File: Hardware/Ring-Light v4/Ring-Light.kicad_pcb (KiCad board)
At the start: 4 copper layers, 124 x 135 mm, 134 parts, among them U1 NCR321PASX, U10 NCR321PASX, U11 NCR321PASX, U12 NCR321PASX, U13 NCR321PASX, U14 NCR321PASX, U15 NCR321PASX, U16 NCR321PASX, U17 NCR321PASX, U18 NCR321PASX, U19 NCR321PASX, U2 NCR321PASX, U20 NCR321PASX, U21 NCR321PASX, U22 NCR321PASX, U23 NCR321PASX, U24 NCR321PASX, U25 NCR321PASX, U26 NCR321PASX, U27 NCR321PASX, U28 NCR321PASX, U29 PCA9685BS,118, U3 NCR321PASX, U30 NCR321PASX, U31 NCR321PASX, U32 NCR321PASX, U33 NCR321PASX, U4 NCR321PASX, U5 NCR321PASX, U6 NCR321PASX, U7 NCR321PASX, U8 NCR321PASX, U9 NCR321PASX

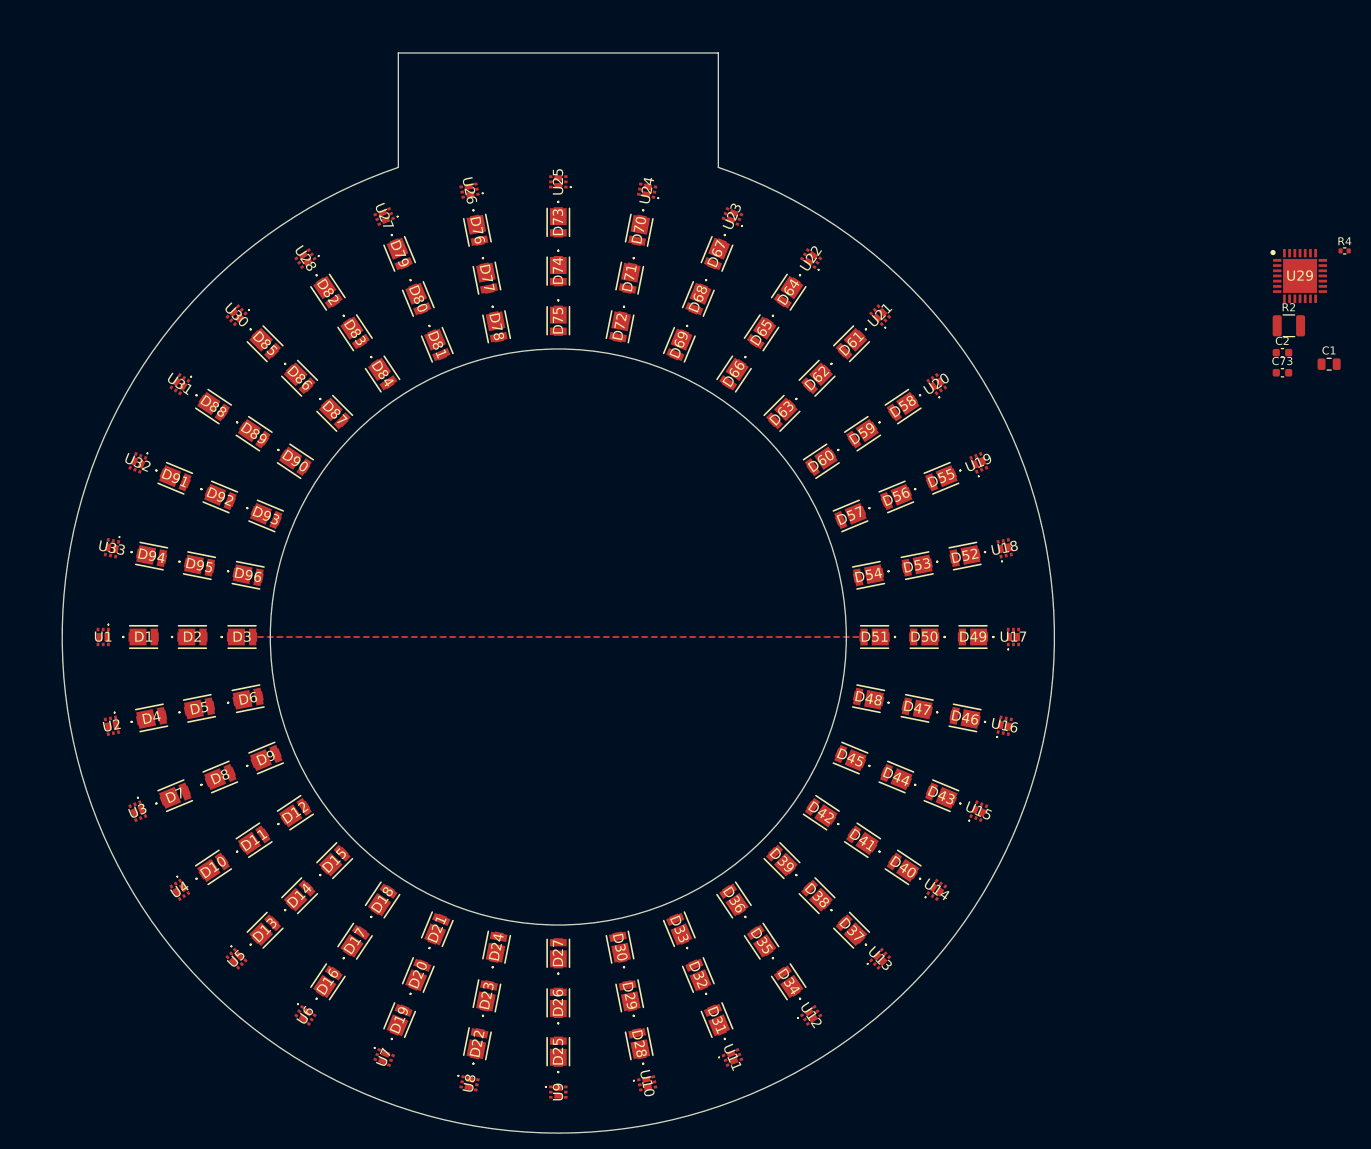
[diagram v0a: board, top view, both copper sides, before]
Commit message: m
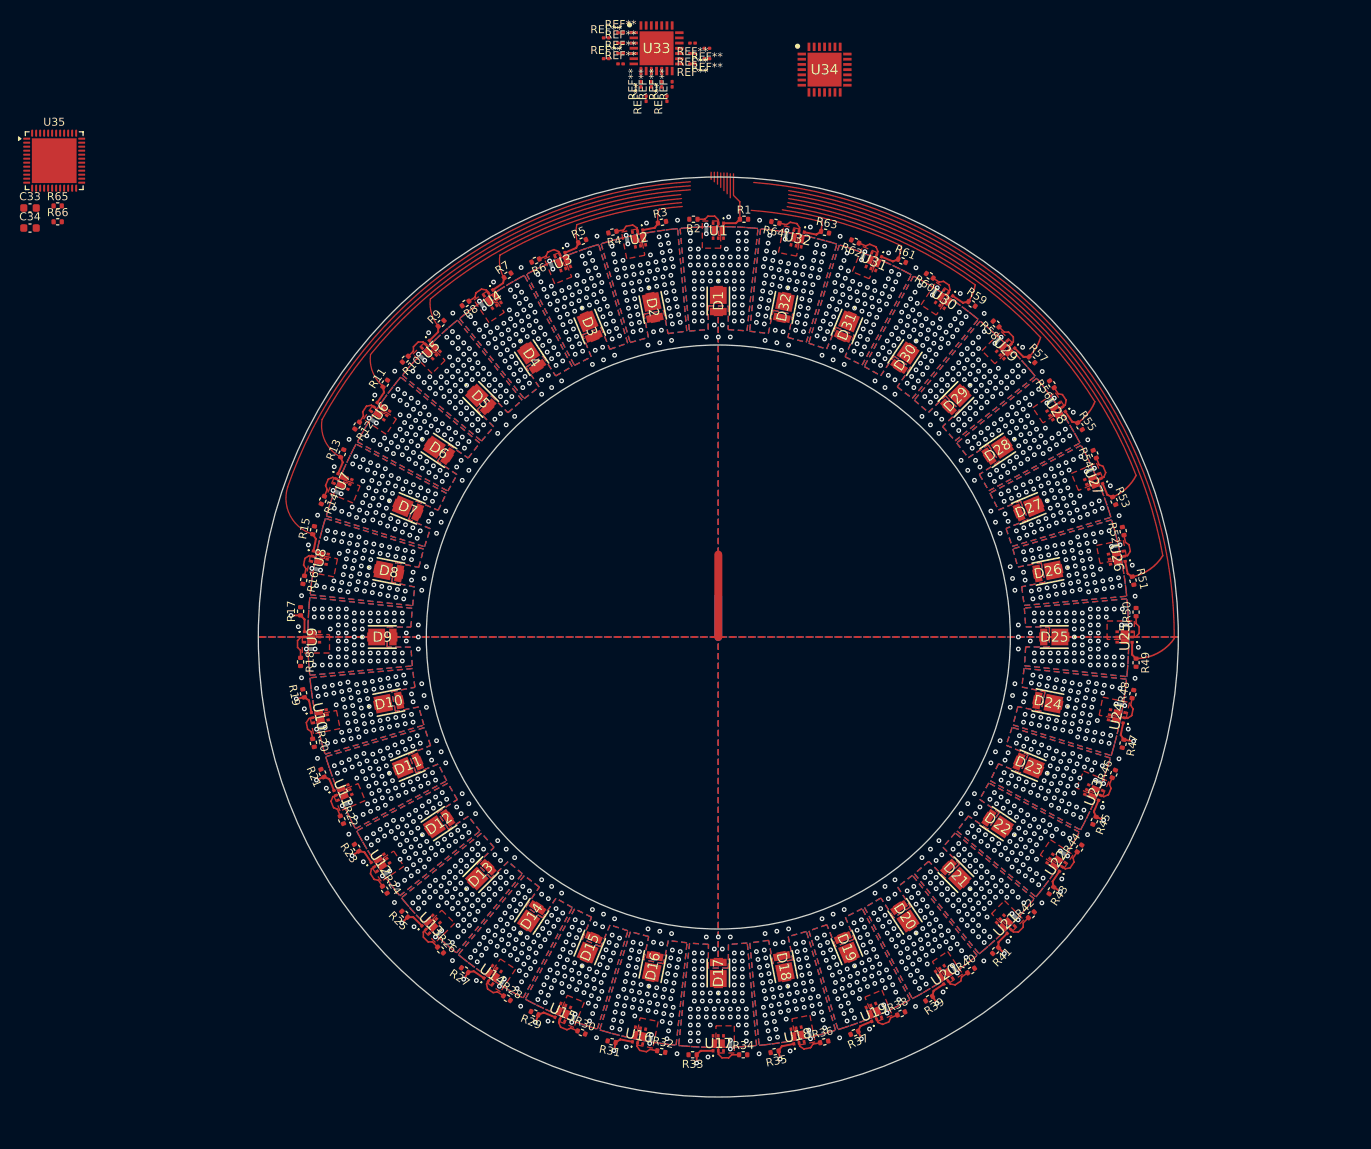
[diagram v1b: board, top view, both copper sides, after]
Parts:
- removed C1: 1uF, Capacitor_SMD:C_0805_2012Metric
- removed C2, C73: 0.1uF, Capacitor_SMD:C_0603_1608Metric
- removed D33, D34, D35, D36, D37, D38, D39, D40, D41, D42, D43, D44, D45, D46, D47, D48, D49, D50, D51, D52, D53, D54, D55, D56, D57, D58, D59, D60, D61, D62, D63, D64, D65, D66, D67, D68, D69, D70, D71, D72, D73, D74, D75, D76, D77, D78, D79, D80, D81, D82, D83, D84, D85, D86, D87, D88, D89, D90, D91, D92, D93, D94, D95, D96: LED, Library:GWJTLRS1EMLVL5XX531
- added C33: 0.1uF, Capacitor_SMD:C_0603_1608Metric, F.Cu at (34.0, 46.4)
- added C34: 0.1uF, Capacitor_SMD:C_0603_1608Metric, F.Cu at (34.0, 48.9)
- added R1: 100k, Resistor_SMD:R_0402_1005Metric, F.Cu at (123.2, 47.8)
- added R10: 9.09, Resistor_SMD:R_0402_1005Metric, F.Cu at (80.9, 65.3)
- added R11: 100k, Resistor_SMD:R_0402_1005Metric, F.Cu at (78.4, 68.3)
- added R12: 9.09, Resistor_SMD:R_0402_1005Metric, F.Cu at (74.9, 73.6)
- added R13: 100k, Resistor_SMD:R_0402_1005Metric, F.Cu at (73.0, 77.1)
- added R14: 9.09, Resistor_SMD:R_0402_1005Metric, F.Cu at (70.6, 82.9)
- added R15: 100k, Resistor_SMD:R_0402_1005Metric, F.Cu at (69.4, 86.7)
- added R16: 9.09, Resistor_SMD:R_0402_1005Metric, F.Cu at (68.2, 92.9)
- added R17: 100k, Resistor_SMD:R_0402_1005Metric, F.Cu at (67.8, 96.8)
- added R18: 9.09, Resistor_SMD:R_0402_1005Metric, F.Cu at (67.8, 103.1)
- added R19: 100k, Resistor_SMD:R_0402_1005Metric, F.Cu at (68.2, 107.0)
- added R20: 9.09, Resistor_SMD:R_0402_1005Metric, F.Cu at (69.4, 113.2)
- added R21: 100k, Resistor_SMD:R_0402_1005Metric, F.Cu at (70.5, 117.0)
- added R22: 9.09, Resistor_SMD:R_0402_1005Metric, F.Cu at (72.9, 122.9)
- added R23: 100k, Resistor_SMD:R_0402_1005Metric, F.Cu at (74.8, 126.3)
- added R24: 9.09, Resistor_SMD:R_0402_1005Metric, F.Cu at (78.3, 131.6)
- added R25: 100k, Resistor_SMD:R_0402_1005Metric, F.Cu at (80.8, 134.7)
- added R26: 9.09, Resistor_SMD:R_0402_1005Metric, F.Cu at (85.3, 139.1)
- added R27: 100k, Resistor_SMD:R_0402_1005Metric, F.Cu at (88.3, 141.6)
- added R28: 9.09, Resistor_SMD:R_0402_1005Metric, F.Cu at (93.6, 145.1)
- added R29: 100k, Resistor_SMD:R_0402_1005Metric, F.Cu at (97.1, 147.0)
- added R3: 100k, Resistor_SMD:R_0402_1005Metric, F.Cu at (113.0, 48.2)
- added R30: 9.09, Resistor_SMD:R_0402_1005Metric, F.Cu at (102.9, 149.4)
- added R31: 100k, Resistor_SMD:R_0402_1005Metric, F.Cu at (106.7, 150.6)
- added R32: 9.09, Resistor_SMD:R_0402_1005Metric, F.Cu at (112.9, 151.8)
- added R33: 100k, Resistor_SMD:R_0402_1005Metric, F.Cu at (116.8, 152.2)
- added R34: 9.09, Resistor_SMD:R_0402_1005Metric, F.Cu at (123.1, 152.2)
- added R35: 100k, Resistor_SMD:R_0402_1005Metric, F.Cu at (127.0, 151.8)
- added R36: 9.09, Resistor_SMD:R_0402_1005Metric, F.Cu at (133.2, 150.6)
- added R37: 100k, Resistor_SMD:R_0402_1005Metric, F.Cu at (137.0, 149.5)
- added R38: 9.09, Resistor_SMD:R_0402_1005Metric, F.Cu at (142.9, 147.1)
- added R39: 100k, Resistor_SMD:R_0402_1005Metric, F.Cu at (146.3, 145.2)
- added R40: 9.09, Resistor_SMD:R_0402_1005Metric, F.Cu at (151.6, 141.7)
- added R41: 100k, Resistor_SMD:R_0402_1005Metric, F.Cu at (154.7, 139.2)
- added R42: 9.09, Resistor_SMD:R_0402_1005Metric, F.Cu at (159.1, 134.7)
- added R43: 100k, Resistor_SMD:R_0402_1005Metric, F.Cu at (161.6, 131.7)
- added R44: 9.09, Resistor_SMD:R_0402_1005Metric, F.Cu at (165.1, 126.4)
- added R45: 100k, Resistor_SMD:R_0402_1005Metric, F.Cu at (167.0, 122.9)
- added R46: 9.09, Resistor_SMD:R_0402_1005Metric, F.Cu at (169.4, 117.1)
- added R47: 100k, Resistor_SMD:R_0402_1005Metric, F.Cu at (170.6, 113.3)
- added R48: 9.09, Resistor_SMD:R_0402_1005Metric, F.Cu at (171.8, 107.1)
- added R49: 100k, Resistor_SMD:R_0402_1005Metric, F.Cu at (172.2, 103.2)
- added R5: 100k, Resistor_SMD:R_0402_1005Metric, F.Cu at (103.0, 50.5)
- added R50: 9.09, Resistor_SMD:R_0402_1005Metric, F.Cu at (172.2, 96.9)
- added R51: 100k, Resistor_SMD:R_0402_1005Metric, F.Cu at (171.8, 93.0)
- added R52: 9.09, Resistor_SMD:R_0402_1005Metric, F.Cu at (170.6, 86.8)
- added R53: 100k, Resistor_SMD:R_0402_1005Metric, F.Cu at (169.5, 83.0)
- added R54: 9.09, Resistor_SMD:R_0402_1005Metric, F.Cu at (167.1, 77.1)
- added R55: 100k, Resistor_SMD:R_0402_1005Metric, F.Cu at (165.2, 73.7)
- added R56: 9.09, Resistor_SMD:R_0402_1005Metric, F.Cu at (161.7, 68.4)
- added R57: 100k, Resistor_SMD:R_0402_1005Metric, F.Cu at (159.2, 65.3)
- added R58: 9.09, Resistor_SMD:R_0402_1005Metric, F.Cu at (154.7, 60.9)
- added R59: 100k, Resistor_SMD:R_0402_1005Metric, F.Cu at (151.7, 58.4)
- added R6: 9.09, Resistor_SMD:R_0402_1005Metric, F.Cu at (97.1, 52.9)
- added R60: 9.09, Resistor_SMD:R_0402_1005Metric, F.Cu at (146.4, 54.9)
- added R61: 100k, Resistor_SMD:R_0402_1005Metric, F.Cu at (142.9, 53.0)
- added R62: 9.09, Resistor_SMD:R_0402_1005Metric, F.Cu at (137.1, 50.6)
- added R63: 100k, Resistor_SMD:R_0402_1005Metric, F.Cu at (133.3, 49.4)
- added R64: 9.09, Resistor_SMD:R_0402_1005Metric, F.Cu at (127.1, 48.2)
- added R65: 10k, Resistor_SMD:R_0402_1005Metric, F.Cu at (37.4, 46.1)
- added R66: 10k, Resistor_SMD:R_0402_1005Metric, F.Cu at (37.4, 48.1)
- added R7: 100k, Resistor_SMD:R_0402_1005Metric, F.Cu at (93.7, 54.8)
- added R8: 9.09, Resistor_SMD:R_0402_1005Metric, F.Cu at (88.4, 58.3)
- added R9: 100k, Resistor_SMD:R_0402_1005Metric, F.Cu at (85.3, 60.8)
- added REF**: R_0201_0603Metric, Resistor_SMD:R_0201_0603Metric, F.Cu at (118.6, 27.7)
- added REF**: R_0201_0603Metric, Resistor_SMD:R_0201_0603Metric, F.Cu at (110.3, 30.9)
- added REF**: R_0201_0603Metric, Resistor_SMD:R_0201_0603Metric, F.Cu at (106.0, 25.1)
- added REF**: R_0201_0603Metric, Resistor_SMD:R_0201_0603Metric, F.Cu at (116.8, 27.1)
- added REF**: R_0201_0603Metric, Resistor_SMD:R_0201_0603Metric, F.Cu at (116.8, 25.8)
- added REF**: R_0201_0603Metric, Resistor_SMD:R_0201_0603Metric, F.Cu at (116.8, 28.4)
- added REF**: R_0201_0603Metric, Resistor_SMD:R_0201_0603Metric, F.Cu at (111.0, 32.7)
- added REF**: R_0201_0603Metric, Resistor_SMD:R_0201_0603Metric, F.Cu at (118.6, 26.4)
- added REF**: R_0201_0603Metric, Resistor_SMD:R_0201_0603Metric, F.Cu at (113.6, 32.7)
- added REF**: R_0201_0603Metric, Resistor_SMD:R_0201_0603Metric, F.Cu at (111.6, 30.9)
- added REF**: R_0201_0603Metric, Resistor_SMD:R_0201_0603Metric, F.Cu at (107.8, 28.4)
- added REF**: R_0201_0603Metric, Resistor_SMD:R_0201_0603Metric, F.Cu at (106.0, 27.7)
- added REF**: R_0201_0603Metric, Resistor_SMD:R_0201_0603Metric, F.Cu at (107.8, 24.5)
- added REF**: R_0201_0603Metric, Resistor_SMD:R_0201_0603Metric, F.Cu at (112.9, 30.9)
- added REF**: R_0201_0603Metric, Resistor_SMD:R_0201_0603Metric, F.Cu at (107.8, 27.1)
- added REF**: R_0201_0603Metric, Resistor_SMD:R_0201_0603Metric, F.Cu at (107.8, 25.8)
- added REF**: R_0201_0603Metric, Resistor_SMD:R_0201_0603Metric, F.Cu at (114.2, 30.9)
- added U34: PCA9685BS,118, Library:QFN65P600X600X100-29N-D, F.Cu at (133.3, 29.1)
- added U35: STM32WB50CGUx, Package_DFN_QFN:QFN-48-1EP_7x7mm_P0.5mm_EP5.6x5.6mm, F.Cu at (37.0, 40.5)
- R2: value 80.6 -> 9.09; footprint Resistor_SMD:R_1210_3225Metric -> Resistor_SMD:R_0402_1005Metric
- R4: value 10k -> 9.09
- U29: value PCA9685BS,118 -> NCR321PASX; footprint Library:QFN65P600X600X100-29N-D -> Library:NCR321PASX
- U33: value NCR321PASX -> PCA9685BS,118; footprint Library:NCR321PASX -> Library:QFN65P600X600X100-29N-D
- moved U28 95.8 mm to (162.2, 71.8)
- moved U27 94.7 mm to (166.9, 80.6)
- moved U26 93.0 mm to (169.8, 90.1)
- moved U33 92.4 mm to (112.3, 26.4), turned to 0 degrees
- moved U1 92.2 mm to (120.0, 49.2)
- moved R4 91.6 mm to (106.8, 49.4), turned to -168.75 degrees
- moved U25 90.8 mm to (170.8, 100.0)
- moved U2 89.7 mm to (110.1, 50.2)
- moved U30 88.5 mm to (148.2, 57.8), turned to 146.25 degrees
- moved D31 88.2 mm to (136.1, 61.2), turned to -112.5 degrees
- moved U24 88.1 mm to (169.8, 109.9)
- moved U31 88.1 mm to (139.4, 53.1), turned to 157.5 degrees
- moved U32 87.1 mm to (129.9, 50.2), turned to 168.75 degrees
- moved U3 86.8 mm to (100.6, 53.1)
- moved D28 86.7 mm to (154.9, 76.7), turned to -146.25 degrees
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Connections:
- D1 pad 1: Net-(D1-K-Pad1) -> /OUT1
- D1 pad 2: Net-(D1-K-Pad1) -> /OUT1
- D1 pad 3: Net-(D1-A-Pad3) -> +12V
- D1 pad 4: Net-(D1-A-Pad3) -> +12V
- D10 pad 1: Net-(D1-K-Pad1) -> /OUT10
- D10 pad 2: Net-(D1-K-Pad1) -> /OUT10
- D10 pad 3: Net-(D1-A-Pad3) -> +12V
- D10 pad 4: Net-(D1-A-Pad3) -> +12V
- D11 pad 1: Net-(D1-A-Pad3) -> /OUT11
- D11 pad 2: Net-(D1-A-Pad3) -> /OUT11
- D11 pad 3: Net-(D2-A-Pad3) -> +12V
- D11 pad 4: Net-(D2-A-Pad3) -> +12V
- D12 pad 1: Net-(D2-A-Pad3) -> /OUT12
- D12 pad 2: Net-(D2-A-Pad3) -> /OUT12
- D13 pad 1: Net-(D1-K-Pad1) -> /OUT13
- D13 pad 2: Net-(D1-K-Pad1) -> /OUT13
- D13 pad 3: Net-(D1-A-Pad3) -> +12V
- D13 pad 4: Net-(D1-A-Pad3) -> +12V
- D14 pad 1: Net-(D1-A-Pad3) -> /OUT14
- D14 pad 2: Net-(D1-A-Pad3) -> /OUT14
- D14 pad 3: Net-(D2-A-Pad3) -> +12V
- D14 pad 4: Net-(D2-A-Pad3) -> +12V
- D15 pad 1: Net-(D2-A-Pad3) -> /OUT15
- D15 pad 2: Net-(D2-A-Pad3) -> /OUT15
- D16 pad 1: Net-(D1-K-Pad1) -> /OUT16
- D16 pad 2: Net-(D1-K-Pad1) -> /OUT16
- D16 pad 3: Net-(D1-A-Pad3) -> +12V
- D16 pad 4: Net-(D1-A-Pad3) -> +12V
- D17 pad 1: Net-(D1-A-Pad3) -> /OUT17
- D17 pad 2: Net-(D1-A-Pad3) -> /OUT17
- D17 pad 3: Net-(D2-A-Pad3) -> +12V
- D17 pad 4: Net-(D2-A-Pad3) -> +12V
- D18 pad 1: Net-(D2-A-Pad3) -> /OUT18
- D18 pad 2: Net-(D2-A-Pad3) -> /OUT18
- D19 pad 1: Net-(D1-K-Pad1) -> /OUT19
- D19 pad 2: Net-(D1-K-Pad1) -> /OUT19
- D19 pad 3: Net-(D1-A-Pad3) -> +12V
- D19 pad 4: Net-(D1-A-Pad3) -> +12V
- D2 pad 1: Net-(D1-A-Pad3) -> /OUT2
- D2 pad 2: Net-(D1-A-Pad3) -> /OUT2
- D2 pad 3: Net-(D2-A-Pad3) -> +12V
- D2 pad 4: Net-(D2-A-Pad3) -> +12V
- D20 pad 1: Net-(D1-A-Pad3) -> /OUT20
- D20 pad 2: Net-(D1-A-Pad3) -> /OUT20
- D20 pad 3: Net-(D2-A-Pad3) -> +12V
- D20 pad 4: Net-(D2-A-Pad3) -> +12V
- D21 pad 1: Net-(D2-A-Pad3) -> /OUT21
- D21 pad 2: Net-(D2-A-Pad3) -> /OUT21
- D22 pad 1: Net-(D1-K-Pad1) -> /OUT22
- D22 pad 2: Net-(D1-K-Pad1) -> /OUT22
- D22 pad 3: Net-(D1-A-Pad3) -> +12V
- D22 pad 4: Net-(D1-A-Pad3) -> +12V
- D23 pad 1: Net-(D1-A-Pad3) -> /OUT23
- D23 pad 2: Net-(D1-A-Pad3) -> /OUT23
- D23 pad 3: Net-(D2-A-Pad3) -> +12V
- D23 pad 4: Net-(D2-A-Pad3) -> +12V
- D24 pad 1: Net-(D2-A-Pad3) -> /OUT24
- D24 pad 2: Net-(D2-A-Pad3) -> /OUT24
- D25 pad 1: Net-(D1-K-Pad1) -> /OUT25
- D25 pad 2: Net-(D1-K-Pad1) -> /OUT25
- D25 pad 3: Net-(D1-A-Pad3) -> +12V
- D25 pad 4: Net-(D1-A-Pad3) -> +12V
- D26 pad 1: Net-(D1-A-Pad3) -> /OUT26
- D26 pad 2: Net-(D1-A-Pad3) -> /OUT26
- D26 pad 3: Net-(D2-A-Pad3) -> +12V
- D26 pad 4: Net-(D2-A-Pad3) -> +12V
- D27 pad 1: Net-(D2-A-Pad3) -> /OUT27
- D27 pad 2: Net-(D2-A-Pad3) -> /OUT27
- D28 pad 1: Net-(D1-K-Pad1) -> /OUT28
- D28 pad 2: Net-(D1-K-Pad1) -> /OUT28
- D28 pad 3: Net-(D1-A-Pad3) -> +12V
- D28 pad 4: Net-(D1-A-Pad3) -> +12V
- D29 pad 1: Net-(D1-A-Pad3) -> /OUT29
- D29 pad 2: Net-(D1-A-Pad3) -> /OUT29
- D29 pad 3: Net-(D2-A-Pad3) -> +12V
- D29 pad 4: Net-(D2-A-Pad3) -> +12V
- D3 pad 1: Net-(D2-A-Pad3) -> /OUT3
- D3 pad 2: Net-(D2-A-Pad3) -> /OUT3
- D30 pad 1: Net-(D2-A-Pad3) -> /OUT30
- D30 pad 2: Net-(D2-A-Pad3) -> /OUT30
- D31 pad 1: Net-(D1-K-Pad1) -> /OUT31
- D31 pad 2: Net-(D1-K-Pad1) -> /OUT31
- D31 pad 3: Net-(D1-A-Pad3) -> +12V
- D31 pad 4: Net-(D1-A-Pad3) -> +12V
- D32 pad 1: Net-(D1-A-Pad3) -> /OUT32
- D32 pad 2: Net-(D1-A-Pad3) -> /OUT32
- D32 pad 3: Net-(D2-A-Pad3) -> +12V
- D32 pad 4: Net-(D2-A-Pad3) -> +12V
- D4 pad 1: Net-(D1-K-Pad1) -> /OUT4
- D4 pad 2: Net-(D1-K-Pad1) -> /OUT4
- D4 pad 3: Net-(D1-A-Pad3) -> +12V
- D4 pad 4: Net-(D1-A-Pad3) -> +12V
- D5 pad 1: Net-(D1-A-Pad3) -> /OUT5
- D5 pad 2: Net-(D1-A-Pad3) -> /OUT5
- D5 pad 3: Net-(D2-A-Pad3) -> +12V
- D5 pad 4: Net-(D2-A-Pad3) -> +12V
- D6 pad 1: Net-(D2-A-Pad3) -> /OUT6
- D6 pad 2: Net-(D2-A-Pad3) -> /OUT6
- D7 pad 1: Net-(D1-K-Pad1) -> /OUT7
- D7 pad 2: Net-(D1-K-Pad1) -> /OUT7
- D7 pad 3: Net-(D1-A-Pad3) -> +12V
- D7 pad 4: Net-(D1-A-Pad3) -> +12V
- D8 pad 1: Net-(D1-A-Pad3) -> /OUT8
- D8 pad 2: Net-(D1-A-Pad3) -> /OUT8
- D8 pad 3: Net-(D2-A-Pad3) -> +12V
- D8 pad 4: Net-(D2-A-Pad3) -> +12V
- D9 pad 1: Net-(D2-A-Pad3) -> /OUT9
- D9 pad 2: Net-(D2-A-Pad3) -> /OUT9
- R2 pad 1: Net-(U1-REXT) -> /REXT1
- R4 pad 1: SDA -> /REXT2
- R4 pad 2: +3.3V -> GND
- U1 pad 1: +12V -> PWM1
- U1 pad 2: Net-(U1-REXT) -> /REXT1
- U1 pad 6: Net-(D1-K-Pad1) -> /OUT1
- U1 pad 7: Net-(D1-K-Pad1) -> /OUT1
- U10 pad 1: +12V -> PWM10
- U10 pad 2: Net-(U1-REXT) -> /REXT10
- U10 pad 3: unconnected-(U1-N/C_1-Pad3) -> unconnected-(U10-N/C_1-Pad3)
- U10 pad 4: unconnected-(U1-N/C_2-Pad4) -> unconnected-(U10-N/C_2-Pad4)
- U10 pad 6: Net-(D1-K-Pad1) -> /OUT10
- U10 pad 7: Net-(D1-K-Pad1) -> /OUT10
- U10 pad 8: unconnected-(U1-N/C_3-Pad8) -> unconnected-(U10-N/C_3-Pad8)
- U11 pad 1: +12V -> PWM11
- U11 pad 2: Net-(U1-REXT) -> /REXT11
- U11 pad 3: unconnected-(U1-N/C_1-Pad3) -> unconnected-(U11-N/C_1-Pad3)
- U11 pad 4: unconnected-(U1-N/C_2-Pad4) -> unconnected-(U11-N/C_2-Pad4)
- U11 pad 6: Net-(D1-K-Pad1) -> /OUT11
- U11 pad 7: Net-(D1-K-Pad1) -> /OUT11
- U11 pad 8: unconnected-(U1-N/C_3-Pad8) -> unconnected-(U11-N/C_3-Pad8)
- U12 pad 1: +12V -> PWM12
- U12 pad 2: Net-(U1-REXT) -> /REXT12
- U12 pad 3: unconnected-(U1-N/C_1-Pad3) -> unconnected-(U12-N/C_1-Pad3)
- U12 pad 4: unconnected-(U1-N/C_2-Pad4) -> unconnected-(U12-N/C_2-Pad4)
- U12 pad 6: Net-(D1-K-Pad1) -> /OUT12
- U12 pad 7: Net-(D1-K-Pad1) -> /OUT12
- U12 pad 8: unconnected-(U1-N/C_3-Pad8) -> unconnected-(U12-N/C_3-Pad8)
- U13 pad 1: +12V -> PWM13
- U13 pad 2: Net-(U1-REXT) -> /REXT13
- U13 pad 3: unconnected-(U1-N/C_1-Pad3) -> unconnected-(U13-N/C_1-Pad3)
- U13 pad 4: unconnected-(U1-N/C_2-Pad4) -> unconnected-(U13-N/C_2-Pad4)
- U13 pad 6: Net-(D1-K-Pad1) -> /OUT13
- U13 pad 7: Net-(D1-K-Pad1) -> /OUT13
- U13 pad 8: unconnected-(U1-N/C_3-Pad8) -> unconnected-(U13-N/C_3-Pad8)
- U14 pad 1: +12V -> PWM14
- U14 pad 2: Net-(U1-REXT) -> /REXT14
- U14 pad 3: unconnected-(U1-N/C_1-Pad3) -> unconnected-(U14-N/C_1-Pad3)
- U14 pad 4: unconnected-(U1-N/C_2-Pad4) -> unconnected-(U14-N/C_2-Pad4)
- U14 pad 6: Net-(D1-K-Pad1) -> /OUT14
- U14 pad 7: Net-(D1-K-Pad1) -> /OUT14
- U14 pad 8: unconnected-(U1-N/C_3-Pad8) -> unconnected-(U14-N/C_3-Pad8)
- U15 pad 1: +12V -> PWM15
- U15 pad 2: Net-(U1-REXT) -> /REXT15
- U15 pad 3: unconnected-(U1-N/C_1-Pad3) -> unconnected-(U15-N/C_1-Pad3)
- U15 pad 4: unconnected-(U1-N/C_2-Pad4) -> unconnected-(U15-N/C_2-Pad4)
- U15 pad 6: Net-(D1-K-Pad1) -> /OUT15
- U15 pad 7: Net-(D1-K-Pad1) -> /OUT15
- U15 pad 8: unconnected-(U1-N/C_3-Pad8) -> unconnected-(U15-N/C_3-Pad8)
- U16 pad 1: +12V -> PWM16
- U16 pad 2: Net-(U1-REXT) -> /REXT16
- U16 pad 3: unconnected-(U1-N/C_1-Pad3) -> unconnected-(U16-N/C_1-Pad3)
- U16 pad 4: unconnected-(U1-N/C_2-Pad4) -> unconnected-(U16-N/C_2-Pad4)
- U16 pad 6: Net-(D1-K-Pad1) -> /OUT16
- U16 pad 7: Net-(D1-K-Pad1) -> /OUT16
- U16 pad 8: unconnected-(U1-N/C_3-Pad8) -> unconnected-(U16-N/C_3-Pad8)
- U17 pad 1: +12V -> PWM17
- U17 pad 2: Net-(U1-REXT) -> /REXT17
- U17 pad 3: unconnected-(U1-N/C_1-Pad3) -> unconnected-(U17-N/C_1-Pad3)
- U17 pad 4: unconnected-(U1-N/C_2-Pad4) -> unconnected-(U17-N/C_2-Pad4)
- U17 pad 6: Net-(D1-K-Pad1) -> /OUT17
- U17 pad 7: Net-(D1-K-Pad1) -> /OUT17
- U17 pad 8: unconnected-(U1-N/C_3-Pad8) -> unconnected-(U17-N/C_3-Pad8)
- U18 pad 1: +12V -> PWM18
- U18 pad 2: Net-(U1-REXT) -> /REXT18
- U18 pad 3: unconnected-(U1-N/C_1-Pad3) -> unconnected-(U18-N/C_1-Pad3)
- U18 pad 4: unconnected-(U1-N/C_2-Pad4) -> unconnected-(U18-N/C_2-Pad4)
- U18 pad 6: Net-(D1-K-Pad1) -> /OUT18
- U18 pad 7: Net-(D1-K-Pad1) -> /OUT18
- U18 pad 8: unconnected-(U1-N/C_3-Pad8) -> unconnected-(U18-N/C_3-Pad8)
- U19 pad 1: +12V -> PWM19
- U19 pad 2: Net-(U1-REXT) -> /REXT19
- U19 pad 3: unconnected-(U1-N/C_1-Pad3) -> unconnected-(U19-N/C_1-Pad3)
- U19 pad 4: unconnected-(U1-N/C_2-Pad4) -> unconnected-(U19-N/C_2-Pad4)
- U19 pad 6: Net-(D1-K-Pad1) -> /OUT19
- U19 pad 7: Net-(D1-K-Pad1) -> /OUT19
- U19 pad 8: unconnected-(U1-N/C_3-Pad8) -> unconnected-(U19-N/C_3-Pad8)
- U2 pad 1: +12V -> PWM2
- U2 pad 2: Net-(U1-REXT) -> /REXT2
- U2 pad 3: unconnected-(U1-N/C_1-Pad3) -> unconnected-(U2-N/C_1-Pad3)
- U2 pad 4: unconnected-(U1-N/C_2-Pad4) -> unconnected-(U2-N/C_2-Pad4)
- U2 pad 6: Net-(D1-K-Pad1) -> /OUT2
- U2 pad 7: Net-(D1-K-Pad1) -> /OUT2
- U2 pad 8: unconnected-(U1-N/C_3-Pad8) -> unconnected-(U2-N/C_3-Pad8)
- U20 pad 1: +12V -> PWM20
- U20 pad 2: Net-(U1-REXT) -> /REXT20
- U20 pad 3: unconnected-(U1-N/C_1-Pad3) -> unconnected-(U20-N/C_1-Pad3)
- U20 pad 4: unconnected-(U1-N/C_2-Pad4) -> unconnected-(U20-N/C_2-Pad4)
- U20 pad 6: Net-(D1-K-Pad1) -> /OUT20
- U20 pad 7: Net-(D1-K-Pad1) -> /OUT20
- U20 pad 8: unconnected-(U1-N/C_3-Pad8) -> unconnected-(U20-N/C_3-Pad8)
- U21 pad 1: +12V -> PWM21
- U21 pad 2: Net-(U1-REXT) -> /REXT21
- U21 pad 3: unconnected-(U1-N/C_1-Pad3) -> unconnected-(U21-N/C_1-Pad3)
- U21 pad 4: unconnected-(U1-N/C_2-Pad4) -> unconnected-(U21-N/C_2-Pad4)
- U21 pad 6: Net-(D1-K-Pad1) -> /OUT21
- U21 pad 7: Net-(D1-K-Pad1) -> /OUT21
- U21 pad 8: unconnected-(U1-N/C_3-Pad8) -> unconnected-(U21-N/C_3-Pad8)
- U22 pad 1: +12V -> PWM22
- U22 pad 2: Net-(U1-REXT) -> /REXT22
- U22 pad 3: unconnected-(U1-N/C_1-Pad3) -> unconnected-(U22-N/C_1-Pad3)
- U22 pad 4: unconnected-(U1-N/C_2-Pad4) -> unconnected-(U22-N/C_2-Pad4)
- U22 pad 6: Net-(D1-K-Pad1) -> /OUT22
- U22 pad 7: Net-(D1-K-Pad1) -> /OUT22
- U22 pad 8: unconnected-(U1-N/C_3-Pad8) -> unconnected-(U22-N/C_3-Pad8)
- U23 pad 1: +12V -> PWM23
- U23 pad 2: Net-(U1-REXT) -> /REXT23
- U23 pad 3: unconnected-(U1-N/C_1-Pad3) -> unconnected-(U23-N/C_1-Pad3)
- U23 pad 4: unconnected-(U1-N/C_2-Pad4) -> unconnected-(U23-N/C_2-Pad4)
- U23 pad 6: Net-(D1-K-Pad1) -> /OUT23
- U23 pad 7: Net-(D1-K-Pad1) -> /OUT23
- U23 pad 8: unconnected-(U1-N/C_3-Pad8) -> unconnected-(U23-N/C_3-Pad8)
- U24 pad 1: +12V -> PWM24
- U24 pad 2: Net-(U1-REXT) -> /REXT24
- U24 pad 3: unconnected-(U1-N/C_1-Pad3) -> unconnected-(U24-N/C_1-Pad3)
- U24 pad 4: unconnected-(U1-N/C_2-Pad4) -> unconnected-(U24-N/C_2-Pad4)
- U24 pad 6: Net-(D1-K-Pad1) -> /OUT24
- U24 pad 7: Net-(D1-K-Pad1) -> /OUT24
- U24 pad 8: unconnected-(U1-N/C_3-Pad8) -> unconnected-(U24-N/C_3-Pad8)
- U25 pad 1: +12V -> PWM25
- U25 pad 2: Net-(U1-REXT) -> /REXT25
- U25 pad 3: unconnected-(U1-N/C_1-Pad3) -> unconnected-(U25-N/C_1-Pad3)
- U25 pad 4: unconnected-(U1-N/C_2-Pad4) -> unconnected-(U25-N/C_2-Pad4)
- U25 pad 6: Net-(D1-K-Pad1) -> /OUT25
- U25 pad 7: Net-(D1-K-Pad1) -> /OUT25
- U25 pad 8: unconnected-(U1-N/C_3-Pad8) -> unconnected-(U25-N/C_3-Pad8)
- U26 pad 1: +12V -> PWM26
- U26 pad 2: Net-(U1-REXT) -> /REXT26
- U26 pad 3: unconnected-(U1-N/C_1-Pad3) -> unconnected-(U26-N/C_1-Pad3)
- U26 pad 4: unconnected-(U1-N/C_2-Pad4) -> unconnected-(U26-N/C_2-Pad4)
- U26 pad 6: Net-(D1-K-Pad1) -> /OUT26
- U26 pad 7: Net-(D1-K-Pad1) -> /OUT26
- U26 pad 8: unconnected-(U1-N/C_3-Pad8) -> unconnected-(U26-N/C_3-Pad8)
- U27 pad 1: +12V -> PWM27
- U27 pad 2: Net-(U1-REXT) -> /REXT27
- U27 pad 3: unconnected-(U1-N/C_1-Pad3) -> unconnected-(U27-N/C_1-Pad3)
- U27 pad 4: unconnected-(U1-N/C_2-Pad4) -> unconnected-(U27-N/C_2-Pad4)
- U27 pad 6: Net-(D1-K-Pad1) -> /OUT27
- U27 pad 7: Net-(D1-K-Pad1) -> /OUT27
- U27 pad 8: unconnected-(U1-N/C_3-Pad8) -> unconnected-(U27-N/C_3-Pad8)
- U28 pad 1: +12V -> PWM28
- U28 pad 2: Net-(U1-REXT) -> /REXT28
- U28 pad 3: unconnected-(U1-N/C_1-Pad3) -> unconnected-(U28-N/C_1-Pad3)
- U28 pad 4: unconnected-(U1-N/C_2-Pad4) -> unconnected-(U28-N/C_2-Pad4)
- U28 pad 6: Net-(D1-K-Pad1) -> /OUT28
- U28 pad 7: Net-(D1-K-Pad1) -> /OUT28
- U28 pad 8: unconnected-(U1-N/C_3-Pad8) -> unconnected-(U28-N/C_3-Pad8)
- U29 pad 1: unconnected-(U29-A3-Pad1) -> PWM29
- U29 pad 2: unconnected-(U29-A4-Pad2) -> /REXT29
- U29 pad 3: PWM1 -> unconnected-(U29-N/C_1-Pad3)
- U29 pad 4: PWM2 -> unconnected-(U29-N/C_2-Pad4)
- U29 pad 5: PWM3 -> GND
- U29 pad 6: PWM4 -> /OUT29
- U29 pad 7: PWM5 -> /OUT29
- U29 pad 8: PWM6 -> unconnected-(U29-N/C_3-Pad8)
- U3 pad 1: +12V -> PWM3
- U3 pad 2: Net-(U1-REXT) -> /REXT3
- U3 pad 3: unconnected-(U1-N/C_1-Pad3) -> unconnected-(U3-N/C_1-Pad3)
- U3 pad 4: unconnected-(U1-N/C_2-Pad4) -> unconnected-(U3-N/C_2-Pad4)
- U3 pad 6: Net-(D1-K-Pad1) -> /OUT3
- U3 pad 7: Net-(D1-K-Pad1) -> /OUT3
- U3 pad 8: unconnected-(U1-N/C_3-Pad8) -> unconnected-(U3-N/C_3-Pad8)
- U30 pad 1: +12V -> PWM30
- U30 pad 2: Net-(U1-REXT) -> /REXT30
- U30 pad 3: unconnected-(U1-N/C_1-Pad3) -> unconnected-(U30-N/C_1-Pad3)
- U30 pad 4: unconnected-(U1-N/C_2-Pad4) -> unconnected-(U30-N/C_2-Pad4)
- U30 pad 6: Net-(D1-K-Pad1) -> /OUT30
- U30 pad 7: Net-(D1-K-Pad1) -> /OUT30
- U30 pad 8: unconnected-(U1-N/C_3-Pad8) -> unconnected-(U30-N/C_3-Pad8)
- U31 pad 1: +12V -> PWM31
- U31 pad 2: Net-(U1-REXT) -> /REXT31
- U31 pad 3: unconnected-(U1-N/C_1-Pad3) -> unconnected-(U31-N/C_1-Pad3)
- U31 pad 4: unconnected-(U1-N/C_2-Pad4) -> unconnected-(U31-N/C_2-Pad4)
- U31 pad 6: Net-(D1-K-Pad1) -> /OUT31
- U31 pad 7: Net-(D1-K-Pad1) -> /OUT31
- U31 pad 8: unconnected-(U1-N/C_3-Pad8) -> unconnected-(U31-N/C_3-Pad8)
- U32 pad 1: +12V -> PWM32
- U32 pad 2: Net-(U1-REXT) -> /REXT32
- U32 pad 3: unconnected-(U1-N/C_1-Pad3) -> unconnected-(U32-N/C_1-Pad3)
- U32 pad 4: unconnected-(U1-N/C_2-Pad4) -> unconnected-(U32-N/C_2-Pad4)
- U32 pad 6: Net-(D1-K-Pad1) -> /OUT32
- U32 pad 7: Net-(D1-K-Pad1) -> /OUT32
- U32 pad 8: unconnected-(U1-N/C_3-Pad8) -> unconnected-(U32-N/C_3-Pad8)
- U33 pad 1: +12V -> unconnected-(U33-A3-Pad1)
- U33 pad 2: Net-(U1-REXT) -> unconnected-(U33-A4-Pad2)
- U33 pad 3: unconnected-(U1-N/C_1-Pad3) -> Net-(U33-LED0)
- U33 pad 4: unconnected-(U1-N/C_2-Pad4) -> Net-(U33-LED1)
- U33 pad 5: GND -> Net-(U33-LED2)
- U33 pad 6: Net-(D1-K-Pad1) -> Net-(U33-LED3)
- U33 pad 7: Net-(D1-K-Pad1) -> Net-(U33-LED4)
- U33 pad 8: unconnected-(U1-N/C_3-Pad8) -> Net-(U33-LED5)
- U4 pad 1: +12V -> PWM4
- U4 pad 2: Net-(U1-REXT) -> /REXT4
- U4 pad 3: unconnected-(U1-N/C_1-Pad3) -> unconnected-(U4-N/C_1-Pad3)
- U4 pad 4: unconnected-(U1-N/C_2-Pad4) -> unconnected-(U4-N/C_2-Pad4)
- U4 pad 6: Net-(D1-K-Pad1) -> /OUT4
- U4 pad 7: Net-(D1-K-Pad1) -> /OUT4
- U4 pad 8: unconnected-(U1-N/C_3-Pad8) -> unconnected-(U4-N/C_3-Pad8)
- U5 pad 1: +12V -> PWM5
- U5 pad 2: Net-(U1-REXT) -> /REXT5
- U5 pad 3: unconnected-(U1-N/C_1-Pad3) -> unconnected-(U5-N/C_1-Pad3)
- U5 pad 4: unconnected-(U1-N/C_2-Pad4) -> unconnected-(U5-N/C_2-Pad4)
- U5 pad 6: Net-(D1-K-Pad1) -> /OUT5
- U5 pad 7: Net-(D1-K-Pad1) -> /OUT5
- U5 pad 8: unconnected-(U1-N/C_3-Pad8) -> unconnected-(U5-N/C_3-Pad8)
- U6 pad 1: +12V -> PWM6
- U6 pad 2: Net-(U1-REXT) -> /REXT6
- U6 pad 3: unconnected-(U1-N/C_1-Pad3) -> unconnected-(U6-N/C_1-Pad3)
- U6 pad 4: unconnected-(U1-N/C_2-Pad4) -> unconnected-(U6-N/C_2-Pad4)
- U6 pad 6: Net-(D1-K-Pad1) -> /OUT6
- U6 pad 7: Net-(D1-K-Pad1) -> /OUT6
- U6 pad 8: unconnected-(U1-N/C_3-Pad8) -> unconnected-(U6-N/C_3-Pad8)
- U7 pad 1: +12V -> PWM7
- U7 pad 2: Net-(U1-REXT) -> /REXT7
- U7 pad 3: unconnected-(U1-N/C_1-Pad3) -> unconnected-(U7-N/C_1-Pad3)
- U7 pad 4: unconnected-(U1-N/C_2-Pad4) -> unconnected-(U7-N/C_2-Pad4)
- U7 pad 6: Net-(D1-K-Pad1) -> /OUT7
- U7 pad 7: Net-(D1-K-Pad1) -> /OUT7
- U7 pad 8: unconnected-(U1-N/C_3-Pad8) -> unconnected-(U7-N/C_3-Pad8)
- U8 pad 1: +12V -> PWM8
- U8 pad 2: Net-(U1-REXT) -> /REXT8
- U8 pad 3: unconnected-(U1-N/C_1-Pad3) -> unconnected-(U8-N/C_1-Pad3)
- U8 pad 4: unconnected-(U1-N/C_2-Pad4) -> unconnected-(U8-N/C_2-Pad4)
- U8 pad 6: Net-(D1-K-Pad1) -> /OUT8
- U8 pad 7: Net-(D1-K-Pad1) -> /OUT8
- U8 pad 8: unconnected-(U1-N/C_3-Pad8) -> unconnected-(U8-N/C_3-Pad8)
- U9 pad 1: +12V -> PWM9
- U9 pad 2: Net-(U1-REXT) -> /REXT9
- U9 pad 3: unconnected-(U1-N/C_1-Pad3) -> unconnected-(U9-N/C_1-Pad3)
- U9 pad 4: unconnected-(U1-N/C_2-Pad4) -> unconnected-(U9-N/C_2-Pad4)
- U9 pad 6: Net-(D1-K-Pad1) -> /OUT9
- U9 pad 7: Net-(D1-K-Pad1) -> /OUT9
- U9 pad 8: unconnected-(U1-N/C_3-Pad8) -> unconnected-(U9-N/C_3-Pad8)
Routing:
- net GND: track 0.00 -> 35.2 mm, vias 0 -> 128
- net PWM1: track 0.00 -> 8.26 mm
- net PWM2: track 0.00 -> 5.31 mm
- net (no net): track 0.00 -> 5.04 mm
- net PWM3: track 0.00 -> 4.98 mm
- net PWM4: track 0.00 -> 4.73 mm
- net PWM5: track 0.00 -> 4.10 mm
- net PWM6: track 0.00 -> 3.88 mm
- net PWM7: track 0.00 -> 3.70 mm
- net PWM9: track 0.00 -> 3.51 mm, vias 0 -> 1
- net PWM24: track 0.00 -> 3.50 mm, vias 0 -> 1
- net /REXT30: track 0.00 -> 3.37 mm
- net /REXT4: track 0.00 -> 3.37 mm
- net /REXT6: track 0.00 -> 3.37 mm
- net /REXT28: track 0.00 -> 3.37 mm
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- added copper zone on B.Cu, net +12V
- added copper zone on In1.Cu, net +12V
- added copper zone on In2.Cu, net +12V
- added copper zone on B.Cu, net /OUT1
- added copper zone on F.Cu, net /OUT1
- added copper zone on In1.Cu, net /OUT1
- added copper zone on In2.Cu, net /OUT1
- added copper zone on B.Cu, net /OUT10
- added copper zone on F.Cu, net /OUT10
- added copper zone on In1.Cu, net /OUT10
- added copper zone on In2.Cu, net /OUT10
- added copper zone on B.Cu, net /OUT11
- added copper zone on F.Cu, net /OUT11
- added copper zone on In1.Cu, net /OUT11
- added copper zone on In2.Cu, net /OUT11
- added copper zone on B.Cu, net /OUT12
- added copper zone on F.Cu, net /OUT12
- added copper zone on In1.Cu, net /OUT12
- added copper zone on In2.Cu, net /OUT12
- added copper zone on B.Cu, net /OUT13
- added copper zone on F.Cu, net /OUT13
- added copper zone on In1.Cu, net /OUT13
- added copper zone on In2.Cu, net /OUT13
- added copper zone on B.Cu, net /OUT14
- added copper zone on F.Cu, net /OUT14
- added copper zone on In1.Cu, net /OUT14
- added copper zone on In2.Cu, net /OUT14
- added copper zone on B.Cu, net /OUT15
- added copper zone on F.Cu, net /OUT15
- added copper zone on In1.Cu, net /OUT15
- added copper zone on In2.Cu, net /OUT15
- added copper zone on B.Cu, net /OUT16
- added copper zone on F.Cu, net /OUT16
- added copper zone on In1.Cu, net /OUT16
- added copper zone on In2.Cu, net /OUT16
- added copper zone on B.Cu, net /OUT17
- added copper zone on F.Cu, net /OUT17
- added copper zone on In1.Cu, net /OUT17
- added copper zone on In2.Cu, net /OUT17
- added copper zone on B.Cu, net /OUT18
- added copper zone on F.Cu, net /OUT18
- added copper zone on In1.Cu, net /OUT18
- added copper zone on In2.Cu, net /OUT18
- added copper zone on B.Cu, net /OUT19
- added copper zone on F.Cu, net /OUT19
- added copper zone on In1.Cu, net /OUT19
- added copper zone on In2.Cu, net /OUT19
- added copper zone on B.Cu, net /OUT2
- added copper zone on F.Cu, net /OUT2
- added copper zone on In1.Cu, net /OUT2
- added copper zone on In2.Cu, net /OUT2
- added copper zone on B.Cu, net /OUT20
- added copper zone on F.Cu, net /OUT20
- added copper zone on In1.Cu, net /OUT20
- added copper zone on In2.Cu, net /OUT20
- added copper zone on B.Cu, net /OUT21
- added copper zone on F.Cu, net /OUT21
- added copper zone on In1.Cu, net /OUT21
- added copper zone on In2.Cu, net /OUT21
- added copper zone on B.Cu, net /OUT22
- added copper zone on F.Cu, net /OUT22
- added copper zone on In1.Cu, net /OUT22
- added copper zone on In2.Cu, net /OUT22
- added copper zone on B.Cu, net /OUT23
- added copper zone on F.Cu, net /OUT23
- added copper zone on In1.Cu, net /OUT23
- added copper zone on In2.Cu, net /OUT23
- added copper zone on B.Cu, net /OUT24
- added copper zone on F.Cu, net /OUT24
- added copper zone on In1.Cu, net /OUT24
- added copper zone on In2.Cu, net /OUT24
- added copper zone on B.Cu, net /OUT25
- added copper zone on F.Cu, net /OUT25
- added copper zone on In1.Cu, net /OUT25
- added copper zone on In2.Cu, net /OUT25
- added copper zone on B.Cu, net /OUT26
- added copper zone on F.Cu, net /OUT26
- added copper zone on In1.Cu, net /OUT26
- added copper zone on In2.Cu, net /OUT26
- added copper zone on B.Cu, net /OUT27
- added copper zone on F.Cu, net /OUT27
- added copper zone on In1.Cu, net /OUT27
- added copper zone on In2.Cu, net /OUT27
- added copper zone on B.Cu, net /OUT28
- added copper zone on F.Cu, net /OUT28
- added copper zone on In1.Cu, net /OUT28
- added copper zone on In2.Cu, net /OUT28
- added copper zone on B.Cu, net /OUT29
- added copper zone on F.Cu, net /OUT29
- added copper zone on In1.Cu, net /OUT29
- added copper zone on In2.Cu, net /OUT29
- added copper zone on B.Cu, net /OUT3
- added copper zone on F.Cu, net /OUT3
- added copper zone on In1.Cu, net /OUT3
- added copper zone on In2.Cu, net /OUT3
- added copper zone on B.Cu, net /OUT30
- added copper zone on F.Cu, net /OUT30
- added copper zone on In1.Cu, net /OUT30
- added copper zone on In2.Cu, net /OUT30
- added copper zone on B.Cu, net /OUT31
- added copper zone on F.Cu, net /OUT31
- added copper zone on In1.Cu, net /OUT31
- added copper zone on In2.Cu, net /OUT31
- added copper zone on B.Cu, net /OUT32
- added copper zone on F.Cu, net /OUT32
- added copper zone on In1.Cu, net /OUT32
- added copper zone on In2.Cu, net /OUT32
- added copper zone on B.Cu, net /OUT4
- added copper zone on F.Cu, net /OUT4
- added copper zone on In1.Cu, net /OUT4
- added copper zone on In2.Cu, net /OUT4
- added copper zone on B.Cu, net /OUT5
- added copper zone on F.Cu, net /OUT5
- added copper zone on In1.Cu, net /OUT5
- added copper zone on In2.Cu, net /OUT5
- added copper zone on B.Cu, net /OUT6
- added copper zone on F.Cu, net /OUT6
- added copper zone on In1.Cu, net /OUT6
- added copper zone on In2.Cu, net /OUT6
- added copper zone on B.Cu, net /OUT7
- added copper zone on F.Cu, net /OUT7
- added copper zone on In1.Cu, net /OUT7
- added copper zone on In2.Cu, net /OUT7
- added copper zone on B.Cu, net /OUT8
- added copper zone on F.Cu, net /OUT8
- added copper zone on In1.Cu, net /OUT8
- added copper zone on In2.Cu, net /OUT8
- added copper zone on B.Cu, net /OUT9
- added copper zone on F.Cu, net /OUT9
- added copper zone on In1.Cu, net /OUT9
- added copper zone on In2.Cu, net /OUT9
- added copper zone on B.Cu, net GND
- added copper zone on F.Cu, net GND
- added copper zone on In1.Cu, net GND
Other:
- board size 124 x 135 mm -> 115 x 115 mm
